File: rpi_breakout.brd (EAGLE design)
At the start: 34.4 x 38.4 mm, 21 parts

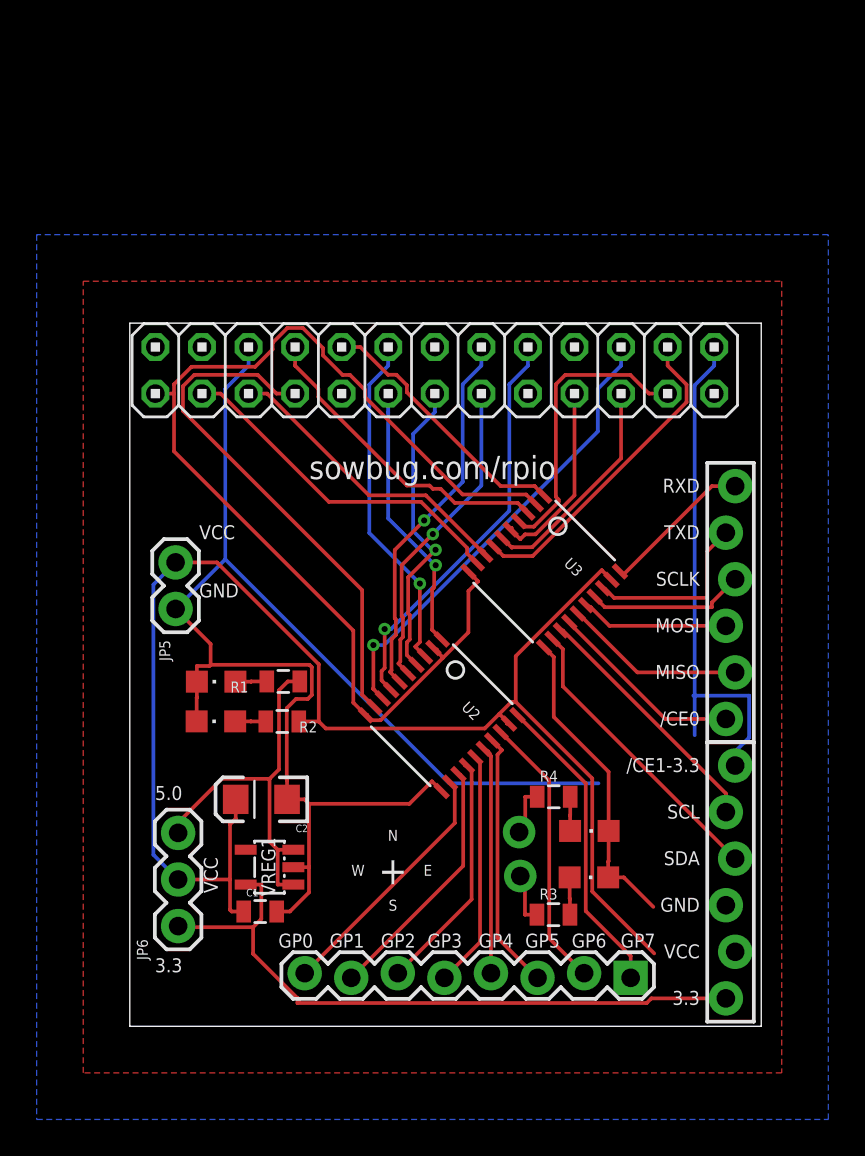
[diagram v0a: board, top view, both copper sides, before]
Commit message: Beefed up everything, made board partial CC size
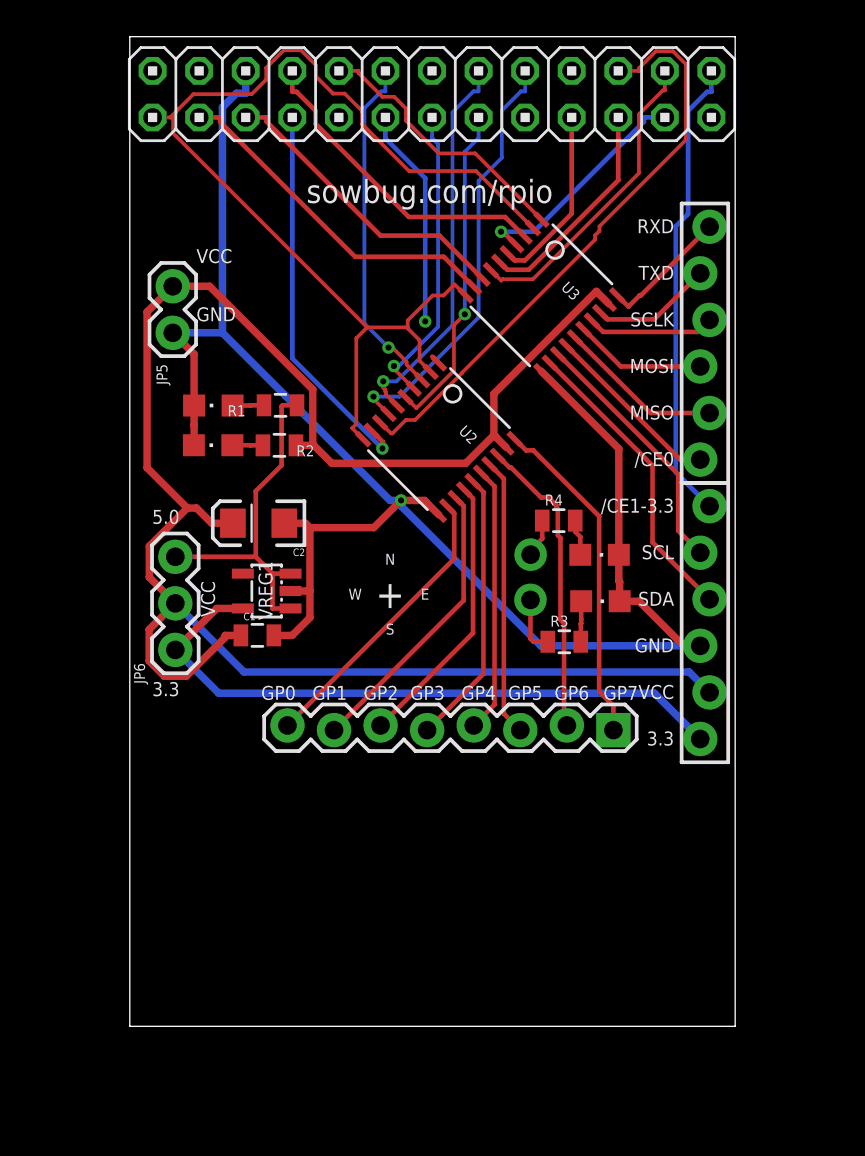
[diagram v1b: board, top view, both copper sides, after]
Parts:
- moved JP8 15.1 mm to (21.9, 25.7)
- moved LED3 15.1 mm to (25.7, 23.2)
- moved LED4 15.1 mm to (25.6, 25.7)
- moved JP7 15.1 mm to (21.9, 23.3)
- moved R4 15.1 mm to (23.4, 27.6)
- moved C1 15.1 mm to (6.96, 21.3)
- moved JP5 15.1 mm to (2.34, 40.4)
- moved JP6 15.1 mm to (2.48, 20.5)
- moved LED1 15.1 mm to (4.56, 33.9)
- moved LED2 15.1 mm to (4.54, 31.7)
- moved R2 15.1 mm to (8.16, 31.7)
- moved U2 15.1 mm to (16.9, 32.0)
- moved VREG1 15.1 mm to (7.47, 23.7)
- moved C2 15.1 mm to (7.03, 27.4)
- moved JP1 15.1 mm to (16.5, 50.8)
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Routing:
- net VCC: track 81.6 -> 101.2 mm
- net GPIO_7: track 28.8 -> 21.3 mm, vias 0 -> 1
- net GPIO_6: track 25.6 -> 32.5 mm, vias 1 -> 0
- net SPI_SCLK: track 16.2 -> 12.8 mm, vias 0 -> 1
- net /SPI_CE1: track 28.8 -> 25.5 mm
- net TXDV: track 9.87 -> 6.66 mm
- net GPIO_0: track 14.8 -> 12.5 mm
- net 3V3_RPI: track 62.1 -> 59.9 mm
- net GPIOV_4: track 13.1 -> 15.1 mm
- net GPIOV_5: track 13.3 -> 15.2 mm
- net GPIOV_6: track 13.9 -> 15.8 mm
- net GPIOV_7: track 14.0 -> 15.9 mm
- net GPIOV_3: track 12.8 -> 14.6 mm
- net SPI_SCLKV: track 8.69 -> 6.95 mm
- net GND: track 97.0 -> 95.3 mm, vias 0 -> 1
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- removed copper zone on layer 1, net GND
- removed copper zone on layer 16, net VCC
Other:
- board size 34.4 x 38.4 mm -> 33 x 54 mm
